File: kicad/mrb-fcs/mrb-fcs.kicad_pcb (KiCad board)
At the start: 2 copper layers, 88.9 x 44.4 mm, 43 parts, among them J1 Phoenix Contact 1988804, J2 USB Mini B Jack, Q1 BSS138K, SW1 FSM4JSMATR, U1 AP63203WU, U2 ESP32-C6-WROOM-1, U3 TLC59284, U4 TLC59284

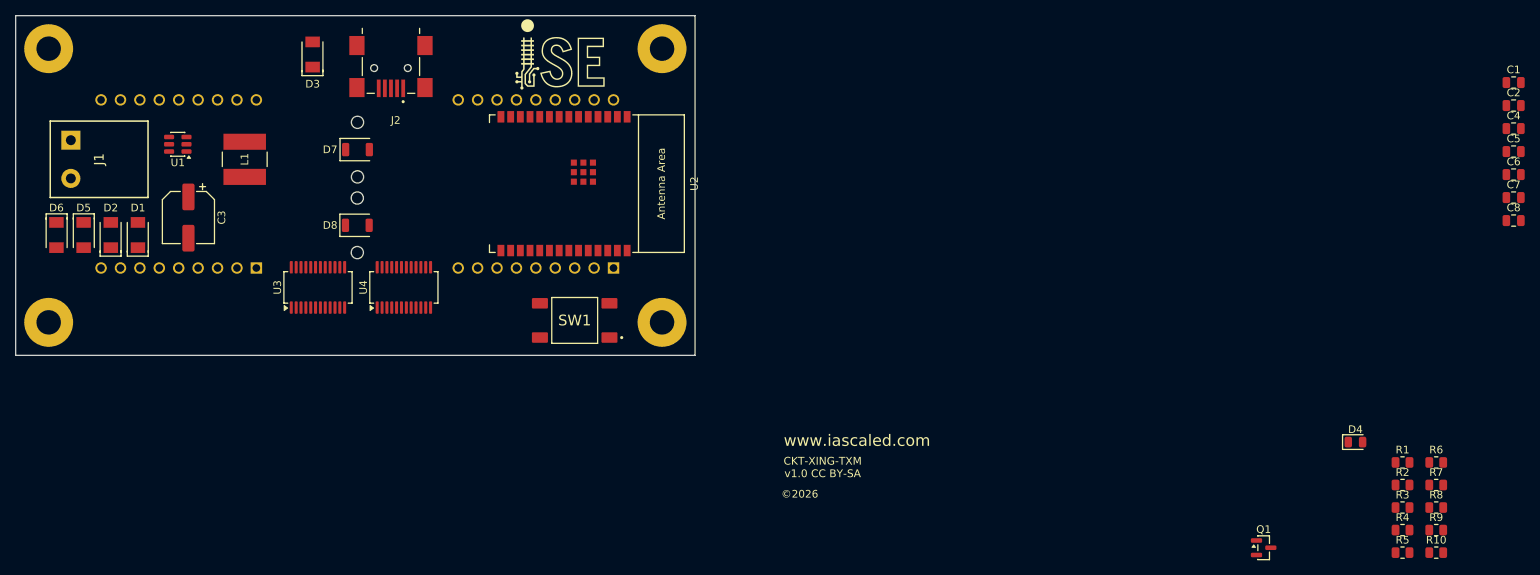
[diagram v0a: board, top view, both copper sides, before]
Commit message: Update schematic, complete PCB
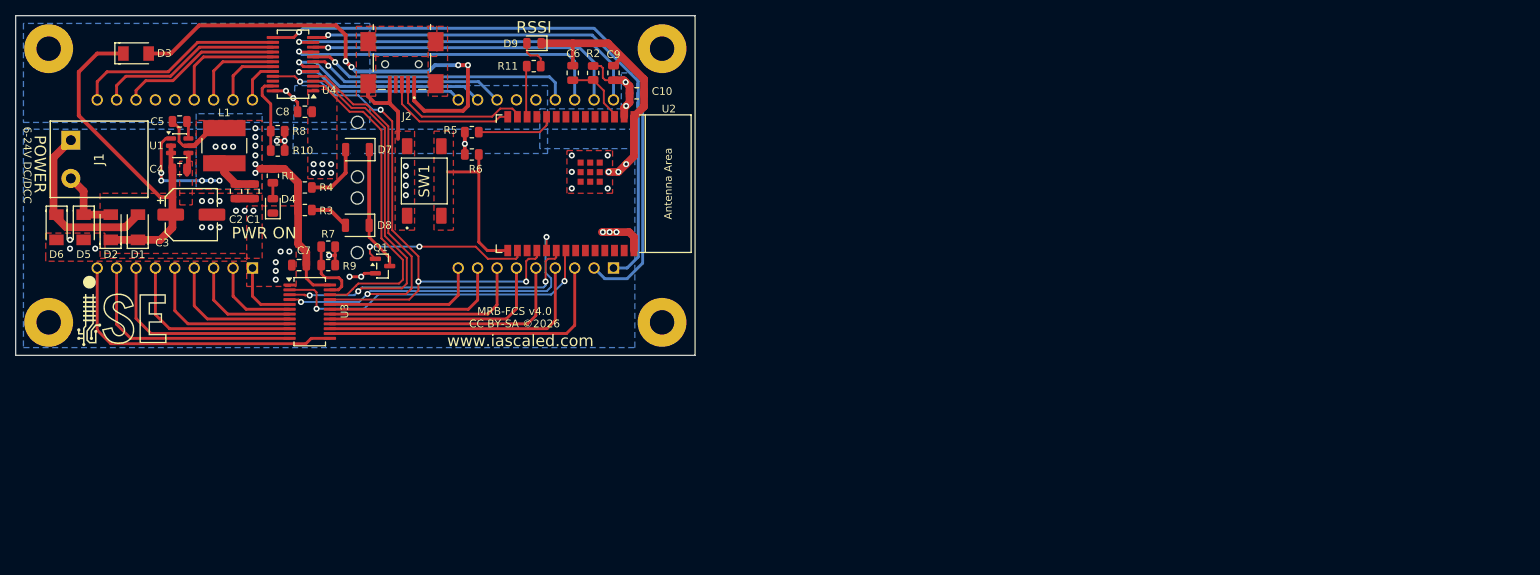
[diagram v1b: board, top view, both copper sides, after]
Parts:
- added C10: 22uF, Capacitor_SMD:C_0805_2012Metric, F.Cu at (106.7, 35.6)
- added C9: 0.1uF, Capacitor_SMD:C_0805_2012Metric, F.Cu at (103.6, 32.9)
- added D9: YELLOW, LED_SMD:LED_0805_2012Metric, F.Cu at (93.2, 29.0)
- added R11: 1k, Resistor_SMD:R_0805_2012Metric, F.Cu at (93.2, 32.0)
- R5, R6: value 1k -> 10k
- moved C4 174.6 mm to (46.9, 45.5)
- moved C5 174.6 mm to (46.9, 39.2)
- moved C2 167.6 mm to (54.2, 48.4), turned to -90 degrees
- moved C1 165.5 mm to (56.5, 48.4), turned to -90 degrees
- moved R10 160.5 mm to (59.7, 43.1)
- moved R8 159.4 mm to (59.7, 40.5)
- moved C7 159.2 mm to (62.5, 58.0), turned to 180 degrees
- moved C8 158.8 mm to (63.2, 38.0)
- moved R1 152.5 mm to (59.1, 46.4), turned to 90 degrees
- moved R4 150.5 mm to (63.2, 47.9), turned to 180 degrees
- moved R9 149.1 mm to (66.3, 58.0)
- moved R3 148.8 mm to (63.2, 50.8), turned to 180 degrees
- moved R7 148.3 mm to (66.3, 55.6)
- moved D4 145.0 mm to (59.1, 50.3), turned to 90 degrees
- moved R5 133.6 mm to (85.1, 40.6), turned to 180 degrees
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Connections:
- net Net-(DISP1-DIG1_C) renamed /DISP1_1_C
- DISP1 pad 1: Net-(DISP1-DIG1_E) -> /DISP1_1_E
- DISP1 pad 10: Net-(DISP1-DIG2_B) -> /DISP1_2_B
- DISP1 pad 11: Net-(DISP1-DIG2_A) -> /DISP1_2_A
- DISP1 pad 12: Net-(DISP1-DIG2_F) -> /DISP1_2_F
- DISP1 pad 15: Net-(DISP1-DIG1_B) -> /DISP1_1_B
- DISP1 pad 16: Net-(DISP1-DIG1_A) -> /DISP1_1_A
- DISP1 pad 17: Net-(DISP1-DIG1_G) -> /DISP1_1_G
- DISP1 pad 18: Net-(DISP1-DIG1_F) -> /DISP1_1_F
- DISP1 pad 2: Net-(DISP1-DIG1_D) -> /DISP1_1_D
- DISP1 pad 4: Net-(DISP1-DIG1_DP) -> /DISP1_1_DP
- DISP1 pad 5: Net-(DISP1-DIG2_E) -> /DISP1_2_E
- DISP1 pad 6: Net-(DISP1-DIG2_D) -> /DISP1_2_D
- DISP1 pad 7: Net-(DISP1-DIG2_G) -> /DISP1_2_G
- DISP1 pad 8: Net-(DISP1-DIG2_C) -> /DISP1_2_C
- DISP1 pad 9: Net-(DISP1-DIG2_DP) -> /DISP1_2_DP
- DISP2 pad 1: Net-(DISP2-DIG1_E) -> /DISP2_1_E
- DISP2 pad 10: Net-(DISP2-DIG2_B) -> /DISP2_2_B
- DISP2 pad 11: Net-(DISP2-DIG2_A) -> /DISP2_2_A
- DISP2 pad 12: Net-(DISP2-DIG2_F) -> /DISP2_2_F
- DISP2 pad 15: Net-(DISP2-DIG1_B) -> /DISP2_1_B
- DISP2 pad 16: Net-(DISP2-DIG1_A) -> /DISP2_1_A
- DISP2 pad 17: Net-(DISP2-DIG1_G) -> /DISP2_1_G
- DISP2 pad 18: Net-(DISP2-DIG1_F) -> /DISP2_1_F
- DISP2 pad 2: Net-(DISP2-DIG1_D) -> /DISP2_1_D
- DISP2 pad 3: Net-(DISP2-DIG1_C) -> /DISP2_1_C
- DISP2 pad 4: Net-(DISP2-DIG1_DP) -> /DISP2_1_DP
- DISP2 pad 5: Net-(DISP2-DIG2_E) -> /DISP2_2_E
- DISP2 pad 6: Net-(DISP2-DIG2_D) -> /DISP2_2_D
- DISP2 pad 7: Net-(DISP2-DIG2_G) -> /DISP2_2_G
- DISP2 pad 8: Net-(DISP2-DIG2_C) -> /DISP2_2_C
- DISP2 pad 9: Net-(DISP2-DIG2_DP) -> /DISP2_2_DP
- U2 pad 12: unconnected-(U2-GPIO11-Pad12) -> Net-(U2-GPIO11)
- U2 pad 16: unconnected-(U2-GPIO18-Pad16) -> /BLINK_COLON
- U2 pad 17: /BLINK_COLON -> unconnected-(U2-GPIO19-Pad17)
- U2 pad 18: Net-(U2-GPIO20) -> /BLANK
- U2 pad 19: Net-(U2-GPIO21) -> /LATCH
- U2 pad 20: Net-(U2-GPIO22) -> /SCLK
- U2 pad 21: Net-(U2-GPIO21) -> /SDO
- U3 pad 10: Net-(DISP1-DIG1_F) -> /DISP1_2_D
- U3 pad 11: Net-(DISP1-DIG1_G) -> /DISP1_2_G
- U3 pad 12: Net-(DISP1-DIG1_DP) -> /DISP1_2_C
- U3 pad 13: Net-(DISP1-DIG2_A) -> /DISP1_2_DP
- U3 pad 14: Net-(DISP1-DIG2_B) -> /DISP2_1_C
- U3 pad 15: Net-(DISP1-DIG2_C) -> /DISP2_1_DP
- U3 pad 16: Net-(DISP1-DIG2_D) -> /DISP2_2_E
- U3 pad 17: Net-(DISP1-DIG2_E) -> /DISP2_2_D
- U3 pad 18: Net-(DISP1-DIG2_F) -> /DISP2_2_G
- U3 pad 19: Net-(DISP1-DIG2_G) -> /DISP2_2_C
- U3 pad 2: Net-(U2-GPIO20) -> /SDO
- U3 pad 20: Net-(DISP1-DIG2_DP) -> /DISP2_2_DP
- U3 pad 21: Net-(U2-GPIO21) -> /BLANK
- U3 pad 3: Net-(U2-GPIO21) -> /SCLK
- U3 pad 4: Net-(U2-GPIO22) -> /LATCH
- U3 pad 5: Net-(DISP1-DIG1_A) -> /DISP1_1_E
- U3 pad 6: Net-(DISP1-DIG1_B) -> /DISP1_1_D
- U3 pad 8: Net-(DISP1-DIG1_D) -> /DISP1_1_DP
- U3 pad 9: Net-(DISP1-DIG1_E) -> /DISP1_2_E
- U4 pad 10: Net-(DISP2-DIG1_F) -> /DISP2_1_G
- U4 pad 11: Net-(DISP2-DIG1_G) -> /DISP2_1_F
- U4 pad 12: Net-(DISP2-DIG1_DP) -> /DISP2_1_E
- U4 pad 13: Net-(DISP2-DIG2_A) -> /DISP2_1_D
- U4 pad 14: Net-(DISP2-DIG2_B) -> /DISP1_2_B
- U4 pad 15: Net-(DISP2-DIG2_C) -> /DISP1_2_A
- U4 pad 16: Net-(DISP2-DIG2_D) -> /DISP1_2_F
- U4 pad 17: Net-(DISP2-DIG2_E) -> /DISP1_1_B
- U4 pad 18: Net-(DISP2-DIG2_F) -> /DISP1_1_A
- U4 pad 19: Net-(DISP2-DIG2_G) -> /DISP1_1_G
- U4 pad 20: Net-(DISP2-DIG2_DP) -> /DISP1_1_F
- U4 pad 21: Net-(U2-GPIO21) -> /BLANK
- U4 pad 3: Net-(U2-GPIO21) -> /SCLK
- U4 pad 4: Net-(U2-GPIO22) -> /LATCH
- U4 pad 5: Net-(DISP2-DIG1_A) -> /DISP2_2_B
- U4 pad 6: Net-(DISP2-DIG1_B) -> /DISP2_2_A
- U4 pad 7: Net-(DISP2-DIG1_C) -> /DISP2_2_F
- U4 pad 8: Net-(DISP2-DIG1_D) -> /DISP2_1_B
- U4 pad 9: Net-(DISP2-DIG1_E) -> /DISP2_1_A
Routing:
- net /LATCH: track 0.00 -> 84.9 mm, vias 0 -> 3
- net /DISP2_1_D: track 0.00 -> 83.7 mm, vias 0 -> 1
- net /SCLK: track 0.00 -> 80.2 mm, vias 0 -> 3
- net /BLANK: track 0.00 -> 72.9 mm, vias 0 -> 4
- net /DISP2_1_E: track 0.00 -> 72.0 mm, vias 0 -> 1
- net GND: track 0.00 -> 68.6 mm, vias 0 -> 43
- net Net-(D3-A): track 0.00 -> 65.9 mm, vias 0 -> 4
- net +3.3V: track 0.00 -> 64.5 mm, vias 0 -> 19
- net /DISP2_1_F: track 0.00 -> 48.9 mm, vias 0 -> 1
- net Net-(D1-K): track 0.00 -> 48.8 mm
- net /SDO: track 0.00 -> 43.8 mm, vias 0 -> 2
- net /DISP2_1_A: track 0.00 -> 43.5 mm, vias 0 -> 1
- net /DISP2_1_G: track 0.00 -> 42.5 mm, vias 0 -> 1
- net Net-(U3-SOUT): track 0.00 -> 42.4 mm
- net /DISP2_1_C: track 0.00 -> 40.0 mm
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- added copper zone on B.Cu, net +3.3V
- added copper zone on F.Cu, net +3.3V
- added copper zone on B.Cu, net GND
- added copper zone on F.Cu, net GND
- added copper zone on F.Cu, net Net-(U2-GPIO9)
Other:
- board text added: "6-24V DC/DCC"
- board text added: "MRB-FCS v4.0 CC BY-SA ©2026"
- board text added: "POWER"
- board text added: "PWR ON"
- board text added: "RSSI"
- board text removed: "CKT-XING-TXM v1.0 CC BY-SA"
- board text removed: "©2026"
